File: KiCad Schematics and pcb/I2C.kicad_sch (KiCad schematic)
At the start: 9 parts, among them J10 Conn_01x04, J11 Conn_01x04, J13 Conn_01x04, SW10 SW_DPDT_x2, SW3 SW_DPDT_x2, SW4 SW_DPDT_x2, SW5 SW_DPDT_x2, SW6 SW_DPDT_x2, SW8 SW_DPDT_x2

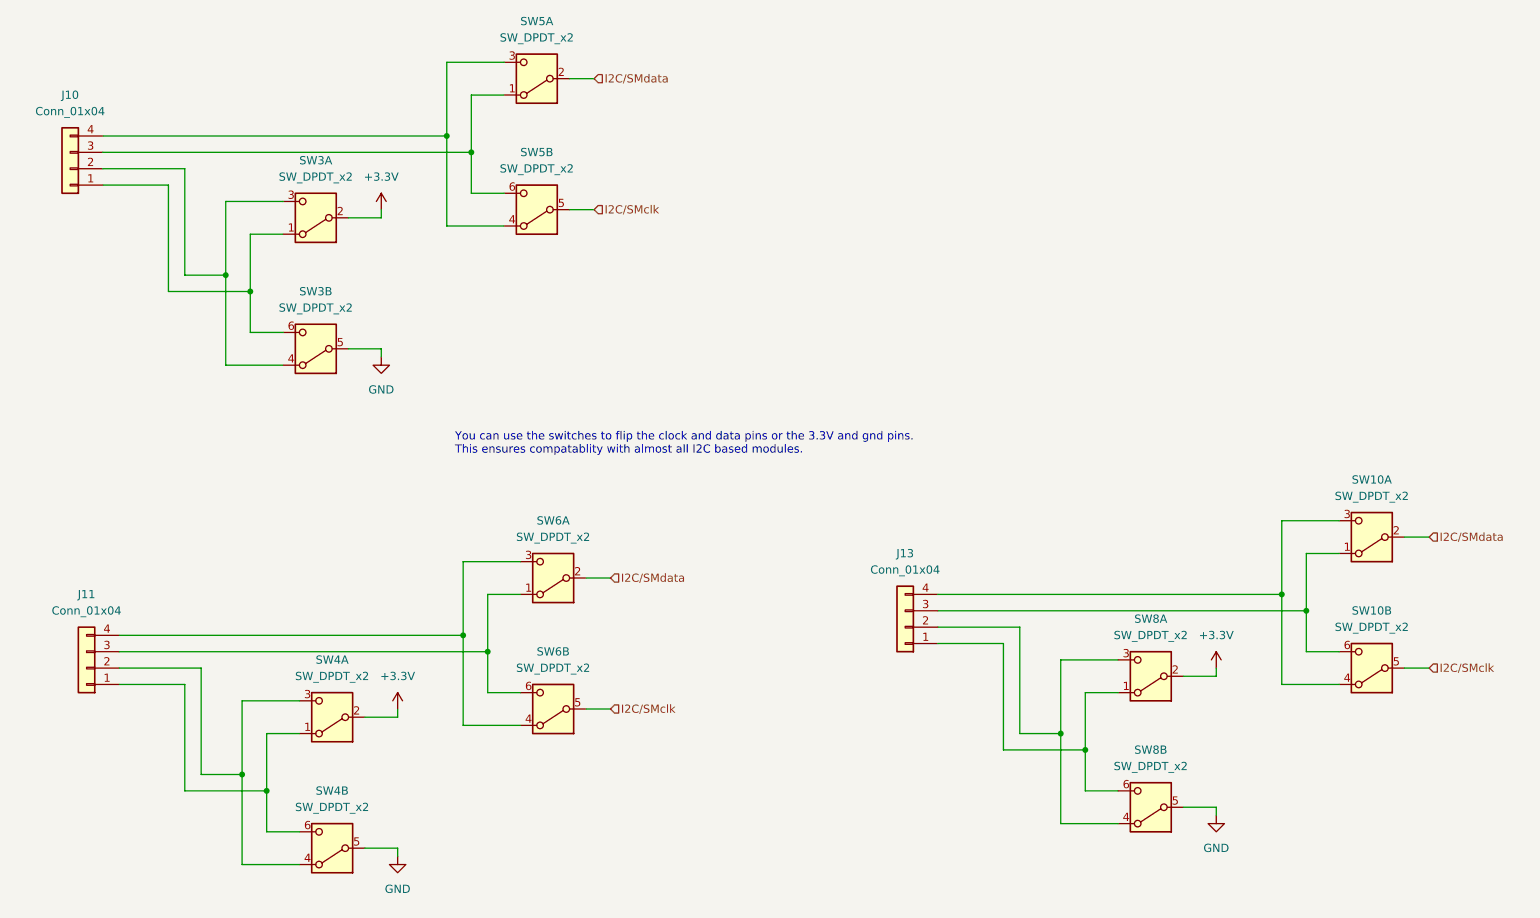
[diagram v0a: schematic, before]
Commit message: v0.1
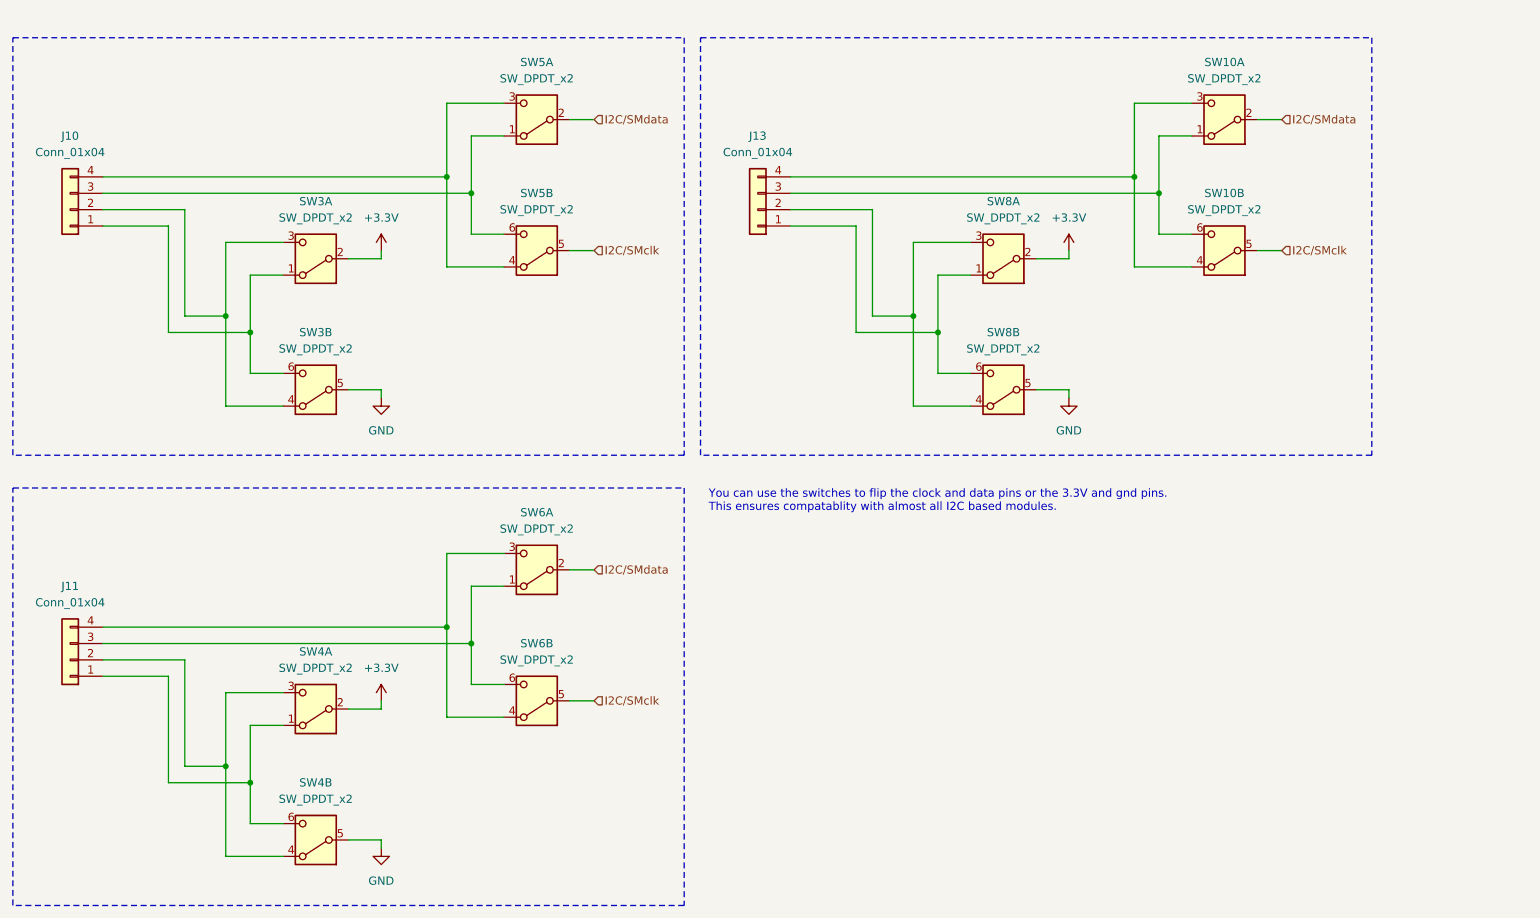
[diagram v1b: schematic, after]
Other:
- moved on the sheet: J10, J11, J13, SW10A, SW10B, SW3A, SW3B, SW4A, SW4B, SW5A, SW5B, SW6A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

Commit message: 0.2
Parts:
- SW10, SW3, SW4, SW5, SW6, SW8: footprint Button_Switch_THT:SW_CuK_JS202011CQN_DPDT_Straight -> ComponentSearch:SW_CK_JS202011CQN_DPDT_Straight
